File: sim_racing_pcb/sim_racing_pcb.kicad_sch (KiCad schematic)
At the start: 21 parts, among them J1 Conn_02x04_Socket, U1 A1302KUA-T, U2 A1302KUA-T, U3 LM358, U4 LM1117MP-3.3, U5 LM7805_TO220, U6 Pico

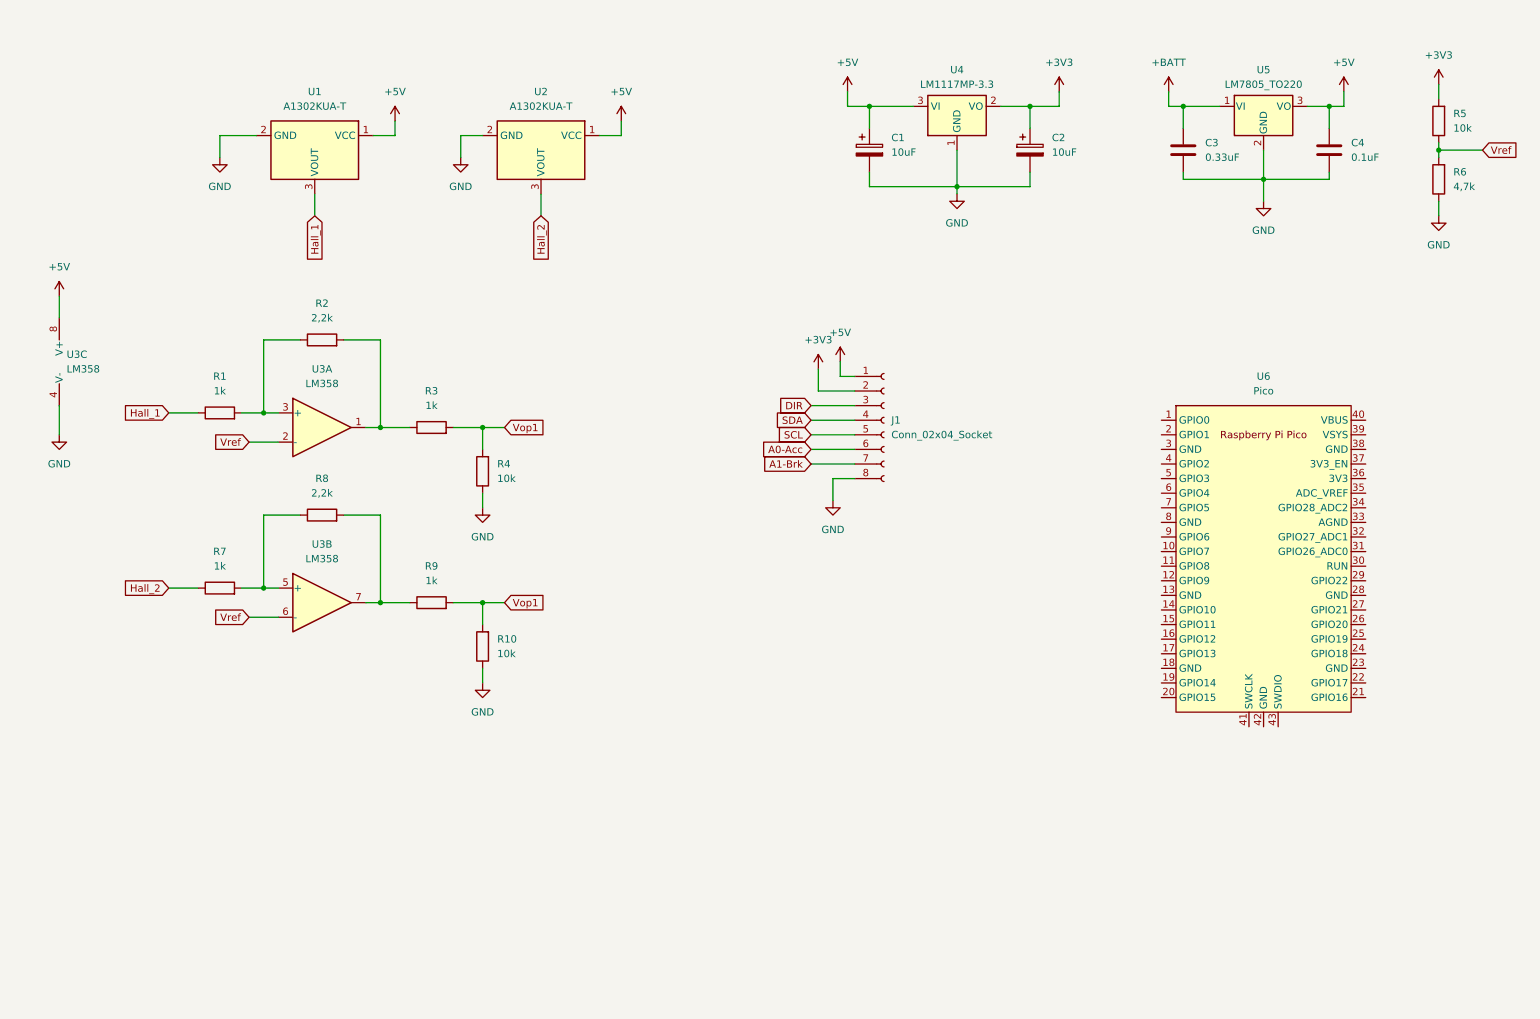
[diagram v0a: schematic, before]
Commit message: codigo de relleno usb lib en C
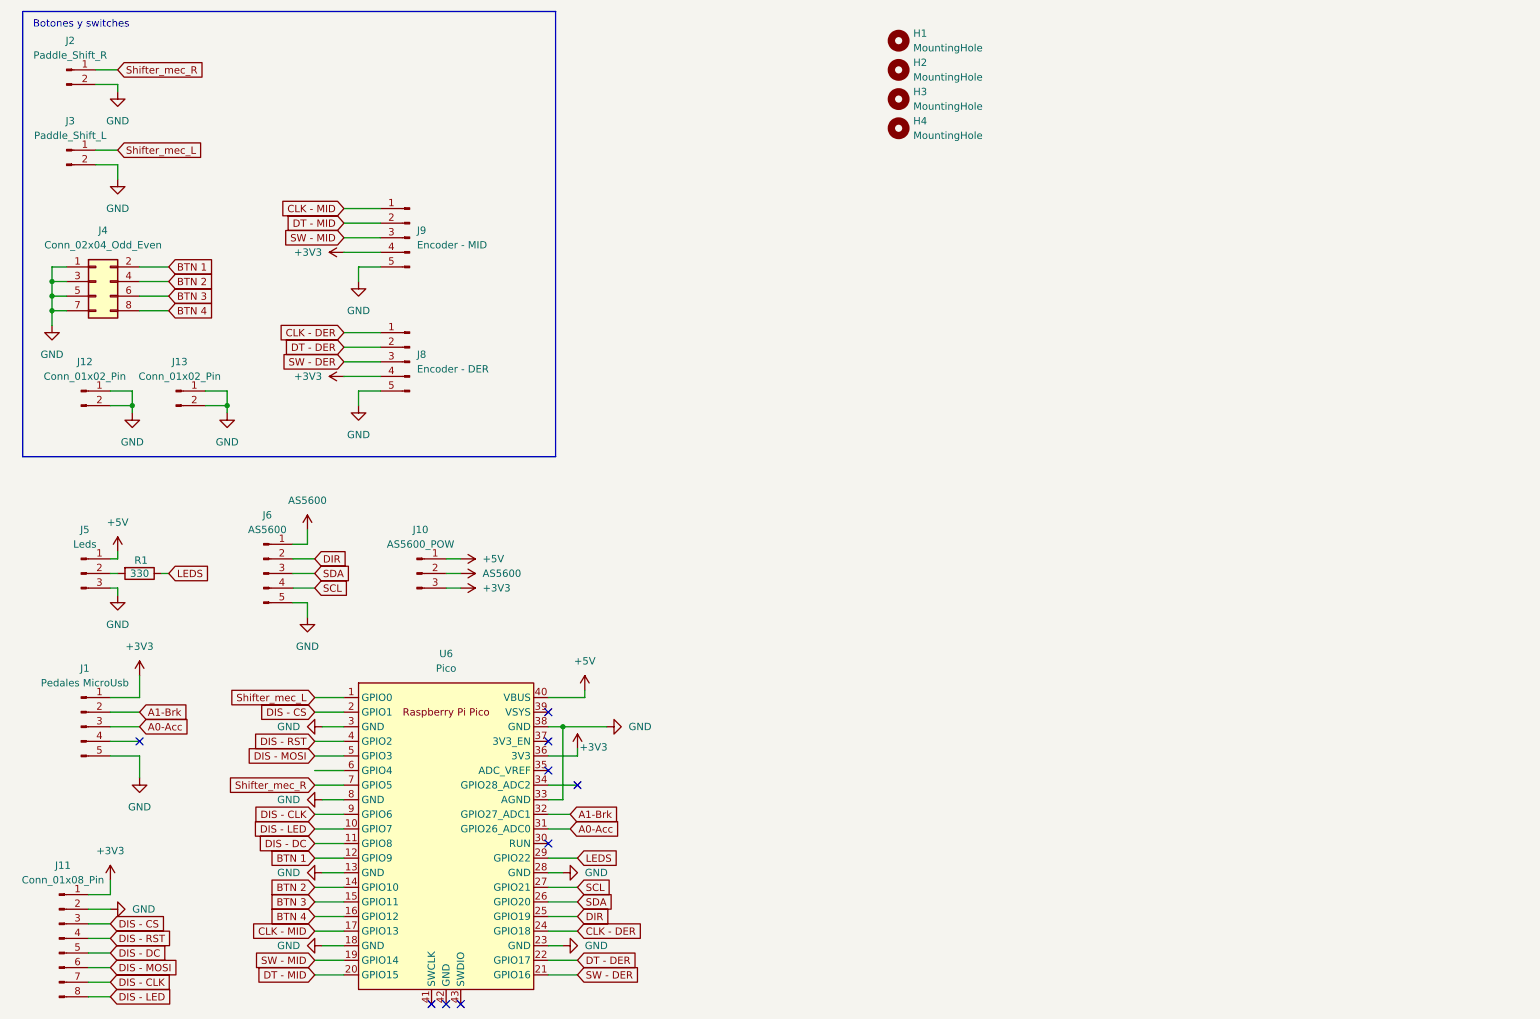
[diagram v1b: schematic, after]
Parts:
- removed C1, C2: 10uF, Capacitor_THT:CP_Radial_D5.0mm_P2.50mm, symbol Device:C_Polarized
- removed C3: 0.33uF, Capacitor_THT:C_Disc_D3.0mm_W2.0mm_P2.50mm, symbol Device:C
- removed C4: 0.1uF, Capacitor_THT:C_Disc_D3.0mm_W2.0mm_P2.50mm, symbol Device:C
- removed J1: Conn_02x04_Socket, Connector_PinHeader_2.54mm:PinHeader_2x04_P2.54mm_Vertical, symbol Connector:Conn_01x08_Socket
- removed R10, R4, R5: 10k, Resistor_THT:R_Axial_DIN0207_L6.3mm_D2.5mm_P10.16mm_Horizontal, symbol Device:R
- removed R2, R8: 2,2k, Resistor_THT:R_Axial_DIN0207_L6.3mm_D2.5mm_P10.16mm_Horizontal, symbol Device:R
- removed R3, R7, R9: 1k, Resistor_THT:R_Axial_DIN0207_L6.3mm_D2.5mm_P10.16mm_Horizontal, symbol Device:R
- removed R6: 4,7k, Resistor_THT:R_Axial_DIN0207_L6.3mm_D2.5mm_P10.16mm_Horizontal, symbol Device:R
- removed U1, U2: A1302KUA-T, Connector_PinHeader_2.54mm:PinHeader_1x03_P2.54mm_Vertical, symbol Sensor_Magnetic:A1302KUA-T
- removed U3: LM358, Package_DIP:DIP-8_W10.16mm_LongPads, symbol Amplifier_Operational:LM358
- removed U4: LM1117MP-3.3, Package_TO_SOT_SMD:SOT-223-3_TabPin2, symbol Regulator_Linear:LM1117MP-3.3
- removed U5: LM7805_TO220, Package_TO_SOT_THT:TO-220-3_Vertical, symbol Regulator_Linear:LM7805_TO220
- added H1, H2, H3, H4: MountingHole, MountingHole:MountingHole_4.3mm_M4_DIN965, symbol Mechanical:MountingHole
- added J1: Pedales MicroUsb, Connector_PinHeader_2.54mm:PinHeader_1x05_P2.54mm_Vertical, symbol Connector:Conn_01x05_Pin
- added J10: AS5600_POW, Connector_PinHeader_2.54mm:PinHeader_1x03_P2.54mm_Vertical, symbol Connector:Conn_01x03_Pin
- added J11: Conn_01x08_Pin, Connector_PinHeader_2.54mm:PinHeader_1x08_P2.54mm_Vertical, symbol Connector:Conn_01x08_Pin
- added J12, J13: Conn_01x02_Pin, Connector_PinHeader_2.54mm:PinHeader_1x02_P2.54mm_Vertical, symbol Connector:Conn_01x02_Pin
- added J2: Paddle_Shift_R, Connector_Molex:Molex_SL_171971-0002_1x02_P2.54mm_Vertical, symbol Connector:Conn_01x02_Pin
- added J3: Paddle_Shift_L, Connector_Molex:Molex_SL_171971-0002_1x02_P2.54mm_Vertical, symbol Connector:Conn_01x02_Pin
- added J4: Conn_02x04_Odd_Even, Connector_PinHeader_2.54mm:PinHeader_2x04_P2.54mm_Vertical, symbol Connector_Generic:Conn_02x04_Odd_Even
- added J5: Leds, Connector_PinHeader_2.54mm:PinHeader_1x03_P2.54mm_Vertical, symbol Connector:Conn_01x03_Pin
- added J6: AS5600, Connector_PinHeader_2.54mm:PinHeader_1x05_P2.54mm_Vertical, symbol Connector:Conn_01x05_Pin
- added J8: Encoder - DER, Connector_PinHeader_2.54mm:PinHeader_1x05_P2.54mm_Vertical, symbol Connector:Conn_01x05_Pin
- added J9: Encoder - MID, Connector_PinHeader_2.54mm:PinHeader_1x05_P2.54mm_Vertical, symbol Connector:Conn_01x05_Pin
- R1: value 1k -> 330
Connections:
- net Hall_1 is gone; now on net LEDS: R1.1
- net +3V3: now also U6.36 (3V3), J1.1 (Pin_1), J10.3 (Pin_3), J11.1 (Pin_1), J8.4 (Pin_4), J9.4 (Pin_4)
- net +5V: now also U6.40 (VBUS), J10.1 (Pin_1), J5.1 (Pin_1)
- net A0-Acc: now also U6.31 (GPIO26_ADC0), J1.3 (Pin_3)
- net A1-Brk: now also U6.32 (GPIO27_ADC1), J1.2 (Pin_2)
- net DIR: now also U6.25 (GPIO19), J6.2 (Pin_2)
- net GND: now also U6.13 (GND), U6.18 (GND), U6.23 (GND), U6.28 (GND), U6.3 (GND), U6.33 (AGND), U6.38 (GND), U6.8 (GND), J1.5 (Pin_5), J11.2 (Pin_2), J12.1 (Pin_1), J12.2 (Pin_2), J13.1 (Pin_1), J13.2 (Pin_2), J2.2 (Pin_2), J3.2 (Pin_2), J4.1 (Pin_1), J4.3 (Pin_3), J4.5 (Pin_5), J4.7 (Pin_7), J5.3 (Pin_3), J6.5 (Pin_5), J8.5 (Pin_5), J9.5 (Pin_5)
- net SCL: now also U6.27 (GPIO21), J6.4 (Pin_4)
- net SDA: now also U6.26 (GPIO20), J6.3 (Pin_3)
- net at R1.2: now also J5.2 (Pin_2)
- net Shifter_mec_L: now reaches U6.1 (GPIO0)
- net Shifter_mec_L: now also J3.1 (Pin_1)
- net DIS - LED: now reaches U6.10 (GPIO7)
- net DIS - LED: now also J11.8 (Pin_8)
- net DIS - DC: now reaches U6.11 (GPIO8)
- net DIS - DC: now also J11.5 (Pin_5)
- net BTN 1: now reaches U6.12 (GPIO9)
- net BTN 1: now also J4.2 (Pin_2)
- net BTN 2: now reaches U6.14 (GPIO10)
- net BTN 2: now also J4.4 (Pin_4)
- net BTN 3: now reaches U6.15 (GPIO11)
- net BTN 3: now also J4.6 (Pin_6)
- net BTN 4: now reaches U6.16 (GPIO12)
- net BTN 4: now also J4.8 (Pin_8)
- net CLK - MID: now reaches U6.17 (GPIO13)
- net CLK - MID: now also J9.1 (Pin_1)
- net SW - MID: now reaches U6.19 (GPIO14)
- net SW - MID: now also J9.3 (Pin_3)
- net DIS - CS: now reaches U6.2 (GPIO1)
- net DIS - CS: now also J11.3 (Pin_3)
- net DT - MID: now reaches U6.20 (GPIO15)
- net DT - MID: now also J9.2 (Pin_2)
- net SW - DER: now reaches U6.21 (GPIO16)
- net SW - DER: now also J8.3 (Pin_3)
- net DT - DER: now reaches U6.22 (GPIO17)
- net DT - DER: now also J8.2 (Pin_2)
- net CLK - DER: now reaches U6.24 (GPIO18)
- net CLK - DER: now also J8.1 (Pin_1)
- net LEDS: now reaches U6.29 (GPIO22)
- net DIS - RST: now reaches U6.4 (GPIO2)
- net DIS - RST: now also J11.4 (Pin_4)
- net DIS - MOSI: now reaches U6.5 (GPIO3)
- net DIS - MOSI: now also J11.6 (Pin_6)
- net Shifter_mec_R: now reaches U6.7 (GPIO5)
- net Shifter_mec_R: now also J2.1 (Pin_1)
- net DIS - CLK: now reaches U6.9 (GPIO6)
- net DIS - CLK: now also J11.7 (Pin_7)
- new net AS5600: J10.2 (Pin_2), J6.1 (Pin_1)
- no-connect marks 0 -> 9
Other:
- note added: "Botones y switches"
- moved on the sheet: U6
